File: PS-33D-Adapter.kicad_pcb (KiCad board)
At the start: 2 copper layers, 17.3 x 14.2 mm, 8 parts, among them J1 CONN_05, J2 Conn_02x04_Counter_Clockwise, Q1 MOSFET-NCH-BSS138, Q2 MOSFET-NCH-BSS138

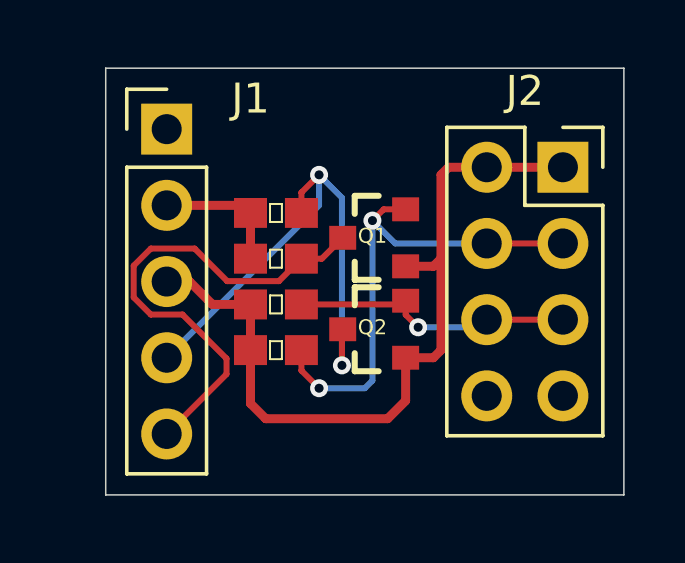
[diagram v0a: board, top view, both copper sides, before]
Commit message: feat: update pcb
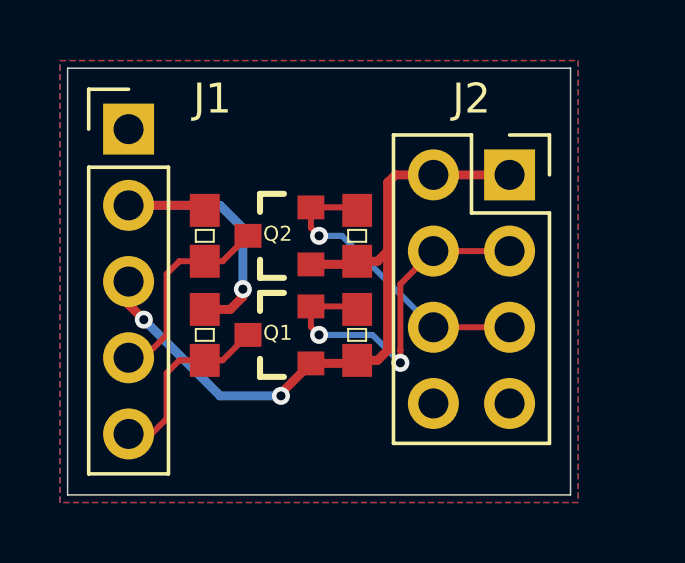
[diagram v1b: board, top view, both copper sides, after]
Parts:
- moved Q1 4.52 mm to (150.9, 83.1)
- moved Q2 4.43 mm to (150.9, 79.8)
- moved R3 3.54 mm to (153.4, 79.8), turned to 90 degrees
- moved R2 3.48 mm to (148.3, 83.1), turned to 270 degrees
- moved R1 2.75 mm to (153.4, 83.1), turned to 90 degrees
- moved R4 2.49 mm to (148.3, 79.8), turned to 270 degrees
- moved J2 1.80 mm to (158.5, 77.7)
- moved J1 1.27 mm to (145.8, 76.2)
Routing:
- net M.SCL: track 17.6 -> 6.85 mm, vias 2 -> 0
- net M.SDA: track 16.6 -> 6.24 mm
- net 5V: track 4.93 -> 10.5 mm, vias 0 -> 1
- net SDA: track 16.7 -> 12.5 mm
- net 3V3: track 26.1 -> 23.8 mm, vias 0 -> 2
- net SCL: track 9.51 -> 10.3 mm
- added copper zone on B.Cu, net GND
- added copper zone on F.Cu, net GND
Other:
- board size 17.3 x 14.2 mm -> 16.8 x 14.2 mm
